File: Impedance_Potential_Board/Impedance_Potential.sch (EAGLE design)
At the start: 80 parts, among them IC1 MAX30001GCWV+, U4 AP2112K-1.8V

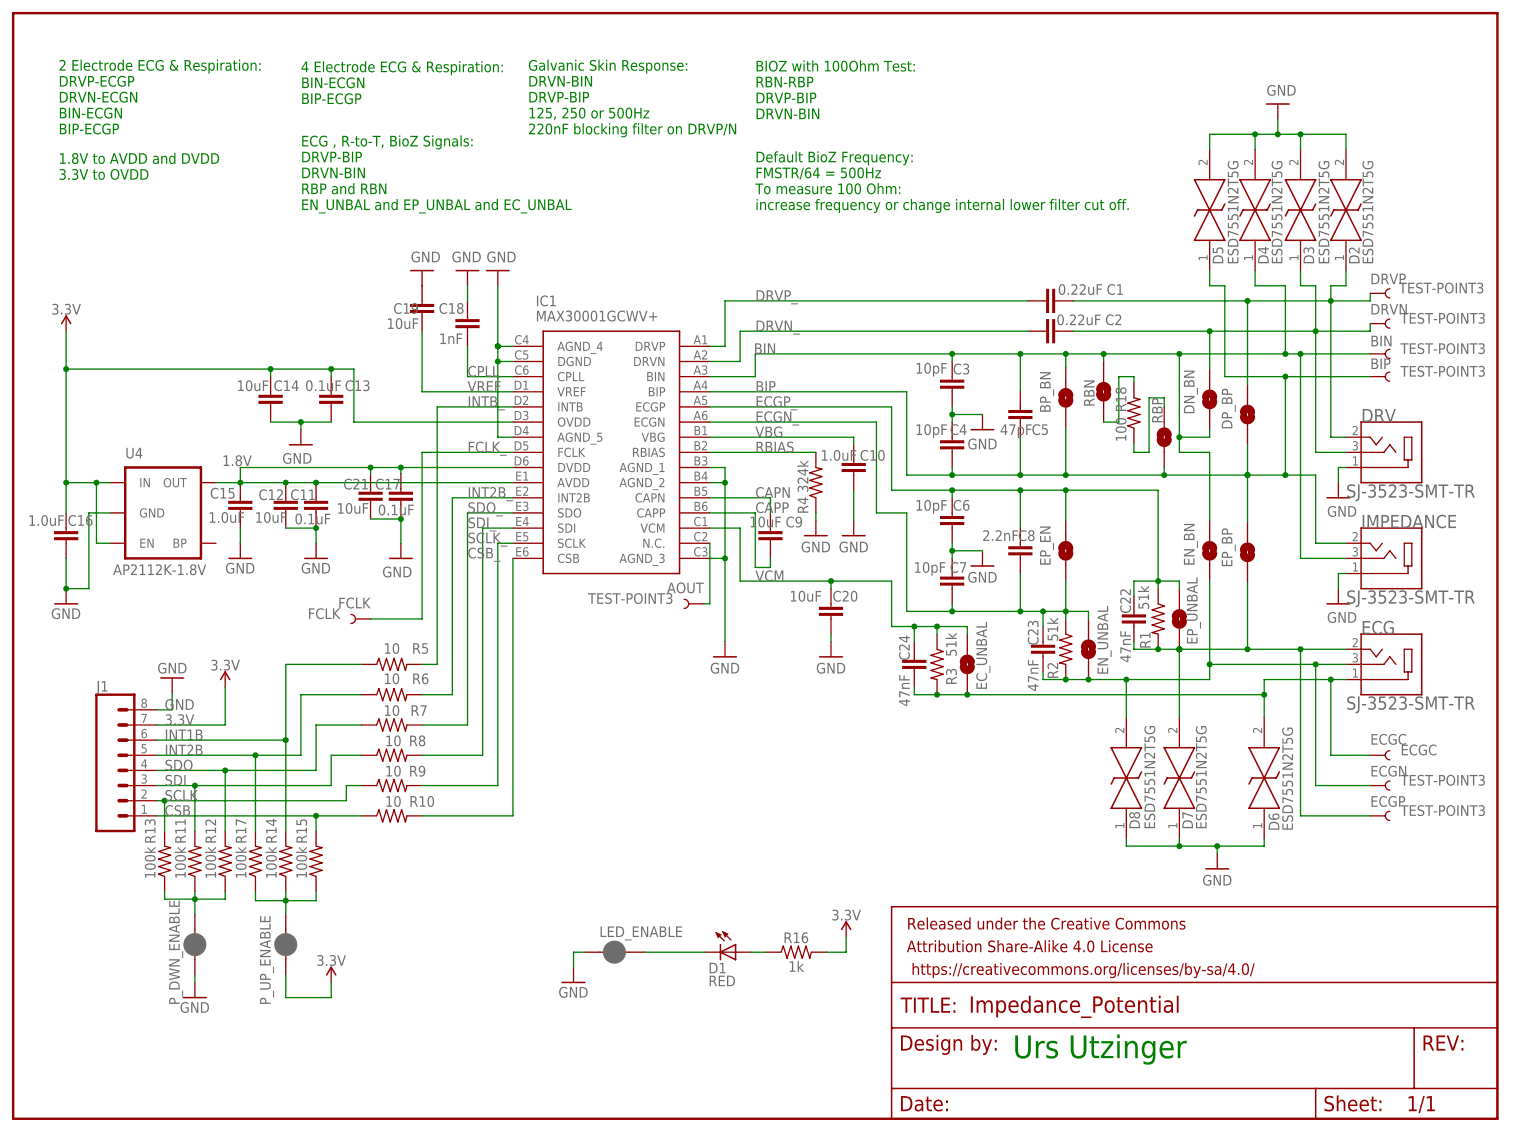
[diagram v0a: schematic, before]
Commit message: CAM Impedance_Potential Board
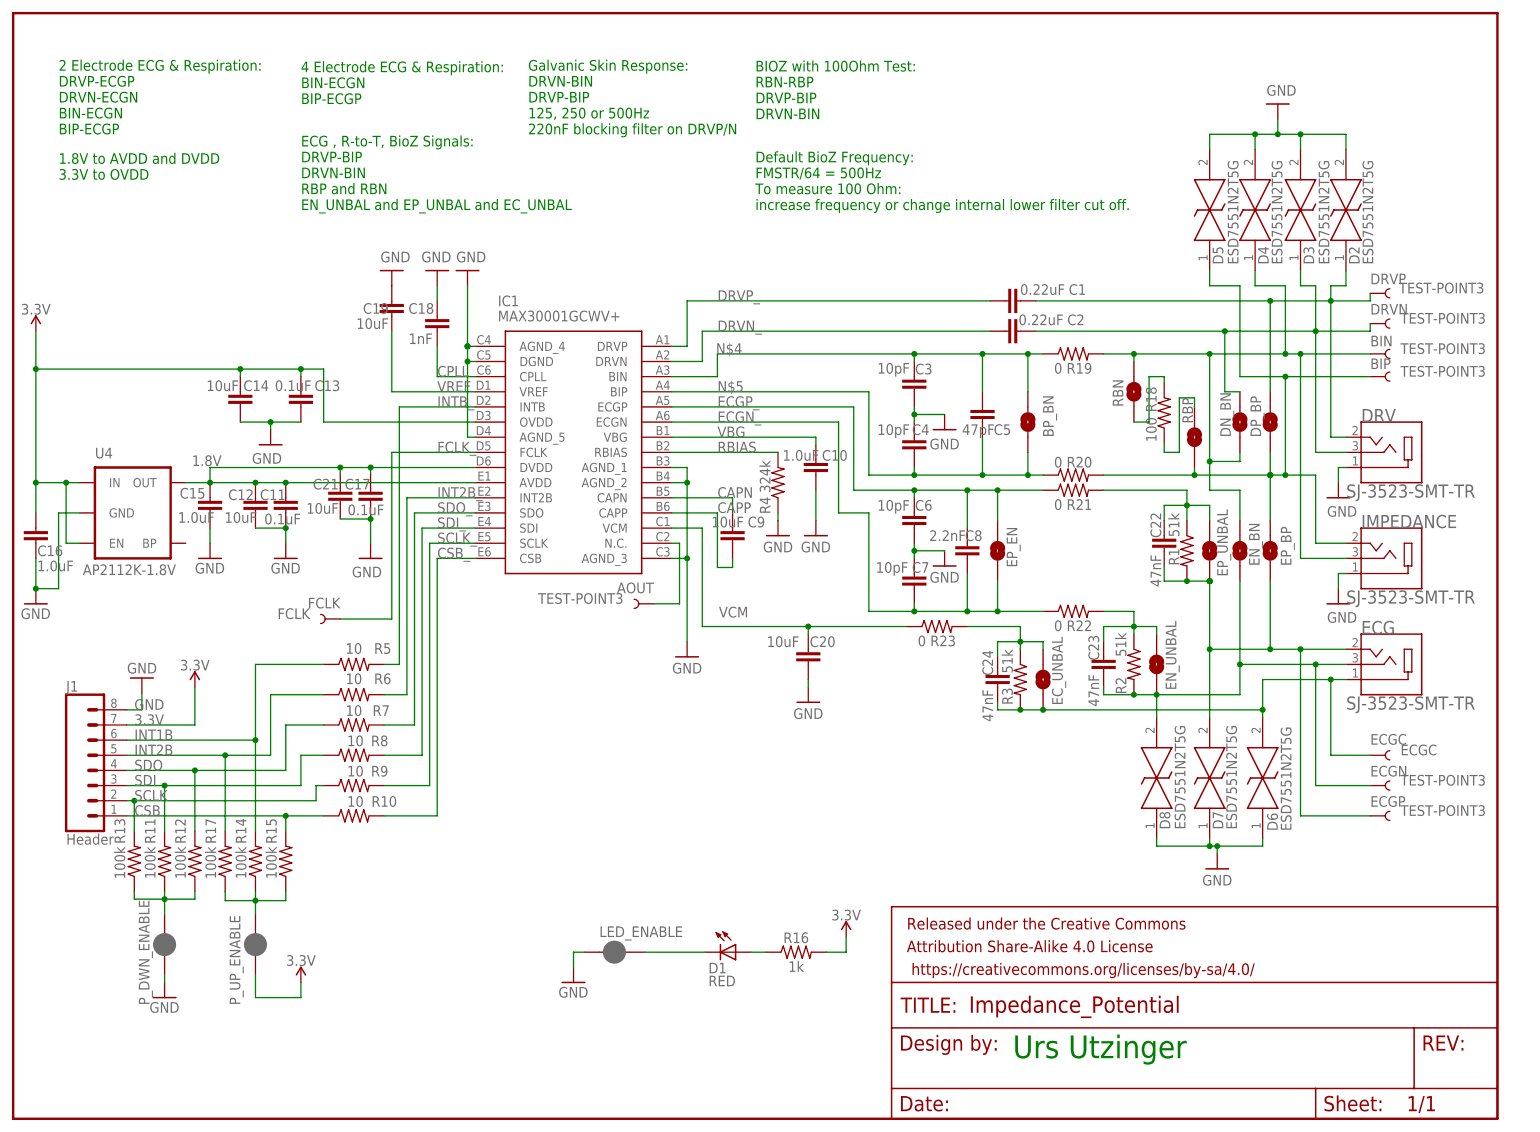
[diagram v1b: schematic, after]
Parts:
- added R19, R20, R21, R22, R23: 0, SparkFun-Resistors:0OHM-0603-1/10W-5%
- J1: value (none) -> Header
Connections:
- new net N$1: C23.1, EN_UNBAL.2, R2.1, R22.2
- new net N$2: C24.1, EC_UNBAL.2, R23.2, R3.1
- new net N$3: C22.1, EP_UNBAL.2, R1.1, R21.2
- new net N$4: BP_BN.2, C3.1, C5.1, IC1.BIN, R19.1
- new net N$5: BP_BN.1, C4.2, C5.2, IC1.BIP, R20.1
- net BIN: now also R19.2; no longer BP_BN.2, C3.1, C5.1, IC1.BIN
- net BIP: now also R20.2; no longer BP_BN.1, C4.2, C5.2, IC1.BIP
- net ECGN_: now also R22.1; no longer C23.1, EN_UNBAL.2, R2.1
- net ECGP_: now also R21.1; no longer C22.1, EP_UNBAL.2, R1.1
- net VCM: now also R23.1; no longer C24.1, EC_UNBAL.2, R3.1
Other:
- moved on the sheet: AOUT, BP_BN, C1, C10, C11, C12, C13, C14, C15, C16, C17, C18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
